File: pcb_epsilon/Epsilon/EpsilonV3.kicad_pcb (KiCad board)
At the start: 2 copper layers, 29 x 11.5 mm, 18 parts, among them J1 SG1m, J2 SG2p, J3 SG1p, J4 SG2m, Q1 AO3401A, U1 ADA4940-1ARZ-R7, U2 DS28E07P+T

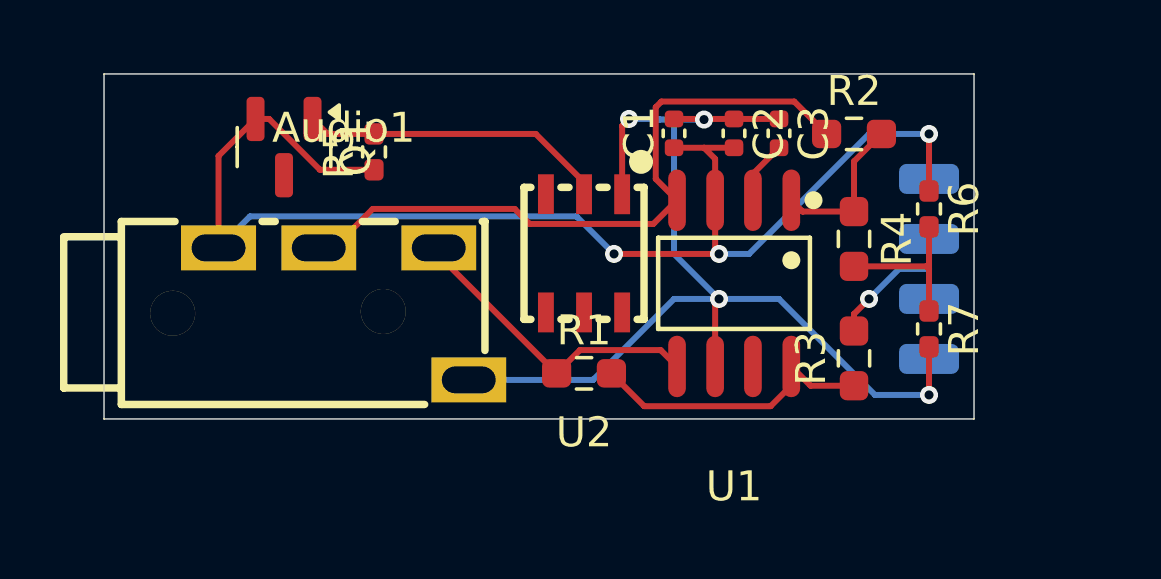
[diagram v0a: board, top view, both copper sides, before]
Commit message: Yolo
Nothing could go wrong
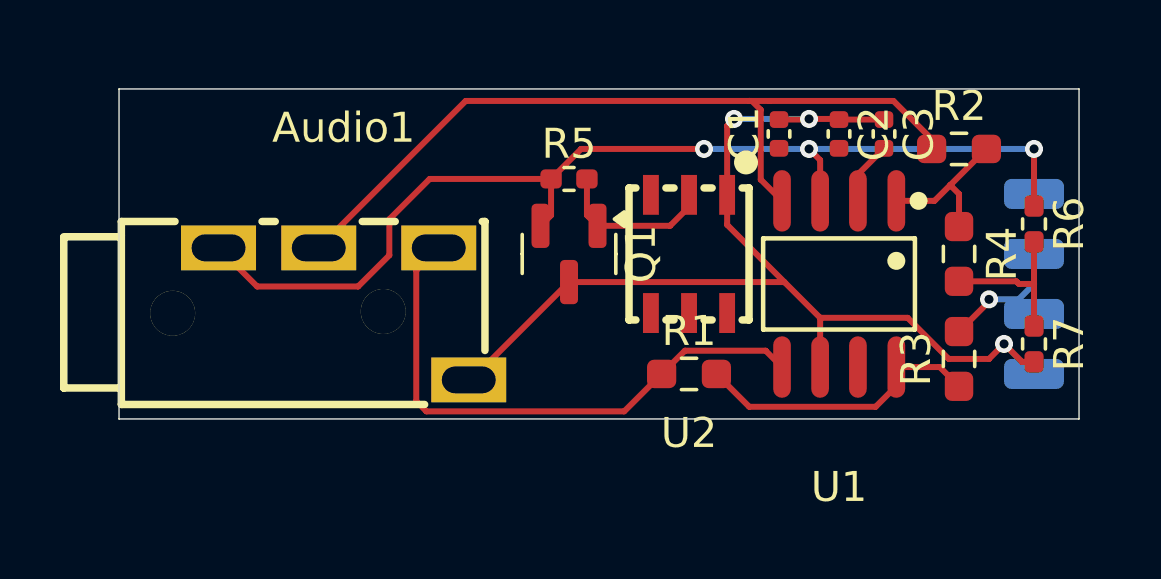
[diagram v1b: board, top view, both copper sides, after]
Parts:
- moved Q1 10.1 mm to (157.0, 126.0)
- moved R5 6.56 mm to (157.0, 123.5), turned to 0 degrees
- moved J1 3.54 mm to (172.5, 126.0)
- moved J2 3.54 mm to (172.5, 128.0)
- moved J3 3.54 mm to (172.5, 124.0)
- moved J4 3.54 mm to (172.5, 130.0)
- moved R2 3.54 mm to (170.0, 122.5)
- moved R4 3.54 mm to (170.0, 126.0)
- moved R6 3.54 mm to (172.5, 125.0)
- moved R7 3.54 mm to (172.5, 129.0)
- moved C1 3.50 mm to (164.0, 122.0)
- moved C2 3.50 mm to (166.0, 122.0)
- moved C3 3.50 mm to (167.5, 122.0)
- moved R1 3.50 mm to (161.0, 130.0)
- moved R3 3.50 mm to (170.0, 129.5)
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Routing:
- net Net-(U1-–OUT): track 10.4 -> 18.8 mm
- net 3V3A_SW: track 44.9 -> 37.3 mm
- net Net-(Q1-G): track 10.3 -> 5.42 mm
- net Net-(U1-+OUT): track 22.6 -> 27.2 mm
- net GND: track 38.1 -> 37.1 mm, vias 4 -> 3
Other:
- board size 29 x 11.5 mm -> 32 x 11 mm
